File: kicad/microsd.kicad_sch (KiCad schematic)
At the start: 3 parts, among them J4 Micro_SD_Card_Det1

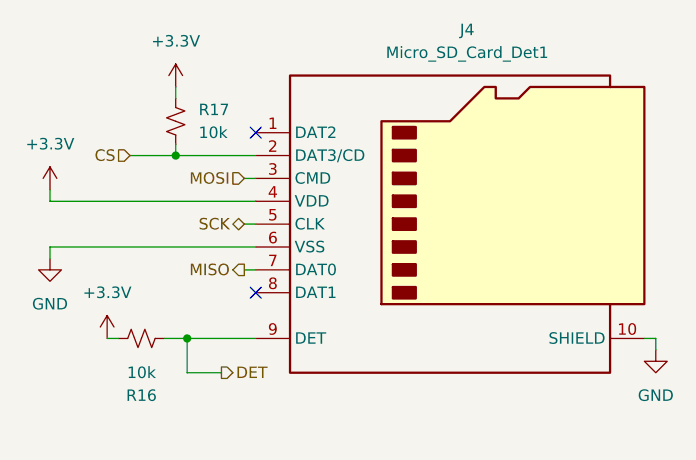
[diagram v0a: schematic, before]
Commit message: finish pcb
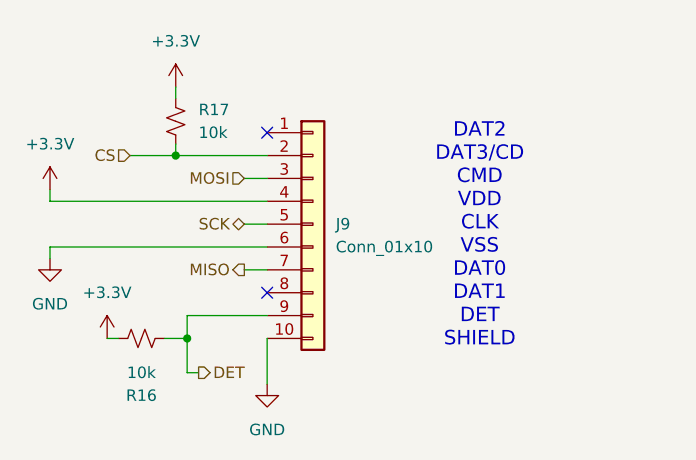
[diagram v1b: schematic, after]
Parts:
- removed J4: Micro_SD_Card_Det1, symbol Connector:Micro_SD_Card_Det1
- added J9: Conn_01x10, Connector_PinSocket_2.54mm:PinSocket_1x10_P2.54mm_Vertical, symbol Connector_Generic:Conn_01x10
- R16, R17: footprint (none) -> Resistor_THT:R_Axial_DIN0207_L6.3mm_D2.5mm_P10.16mm_Horizontal
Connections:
- net +3.3V: now also J9.4 (Pin_4)
- net CS: now also J9.2 (Pin_2)
- net DET: now also J9.9 (Pin_9)
- net GND: now also J9.10 (Pin_10), J9.6 (Pin_6)
- net MISO: now also J9.7 (Pin_7)
- net MOSI: now also J9.3 (Pin_3)
- net SCK: now also J9.5 (Pin_5)
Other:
- note added: "DAT2 DAT3/CD CMD VDD CLK VSS DAT0 DAT1 DET SHIELD"
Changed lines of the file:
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@@
 	(generator_version "9.0")
 	(paper "A4")
+	(text "DAT2\nDAT3/CD\nCMD\nVDD\nCLK\nVSS\nDAT0\nDAT1\nDET\nSHIELD"
+		(exclude_from_sim no)
+		(at 238.252 59.69 0)
+		(effects
+			(font
+				(size 1.6002 1.6002)
+			)
+		)
+	)
 	(junction
 		(at 204.47 50.8)
@@
 	)
 	(no_connect
-		(at 213.36 48.26)
+		(at 214.63 48.26)
 	)
 	(no_connect
-		(at 213.36 66.04)
-	)
-	(wire
-		(pts
-			(xy 257.81 71.12) (xy 256.54 71.12)
-		)
-		(stroke
-			(width 0)
-			(type default)
-		)
-	)
-	(wire
-		(pts
-			(xy 190.5 60.96) (xy 213.36 60.96)
+		(at 214.63 66.04)
+	)
+	(wire
+		(pts
+			(xy 190.5 60.96) (xy 214.63 60.96)
+		)
+		(stroke
+			(width 0)
+			(type default)
+		)
+	)
+	(wire
+		(pts
+			(xy 205.74 68.58) (xy 205.74 71.12)
 		)
 		(stroke
@@
 	(wire
 		(pts
-			(xy 204.47 50.8) (xy 213.36 50.8)
+			(xy 204.47 50.8) (xy 214.63 50.8)
 		)
 		(stroke
@@
 	(wire
 		(pts
-			(xy 212.09 58.42) (xy 213.36 58.42)
-		)
-		(stroke
-			(width 0)
-			(type default)
-		)
-	)
-	(wire
-		(pts
-			(xy 190.5 55.88) (xy 213.36 55.88)
-		)
-		(stroke
-			(width 0)
-			(type default)
-		)
-	)
-	(wire
-		(pts
-			(xy 257.81 72.39) (xy 257.81 71.12)
-		)
-		(stroke
-			(width 0)
-			(type default)
-		)
-	)
-	(wire
-		(pts
-			(xy 212.09 63.5) (xy 213.36 63.5)
+			(xy 212.09 58.42) (xy 214.63 58.42)
+		)
+		(stroke
+			(width 0)
+			(type default)
+		)
+	)
+	(wire
+		(pts
+			(xy 190.5 55.88) (xy 214.63 55.88)
+		)
+		(stroke
+			(width 0)
+			(type default)
+		)
+	)
+	(wire
+		(pts
+			(xy 212.09 63.5) (xy 214.63 63.5)
 		)
 		(stroke
@@
 	(wire
 		(pts
-			(xy 209.55 74.93) (xy 205.74 74.93)
-		)
-		(stroke
-			(width 0)
-			(type default)
-		)
-	)
-	(wire
-		(pts
-			(xy 205.74 71.12) (xy 213.36 71.12)
+			(xy 207.01 74.93) (xy 205.74 74.93)
+		)
+		(stroke
+			(width 0)
+			(type default)
+		)
+	)
+	(wire
+		(pts
+			(xy 214.63 71.12) (xy 214.63 76.2)
+		)
+		(stroke
+			(width 0)
+			(type default)
+		)
+	)
+	(wire
+		(pts
+			(xy 205.74 68.58) (xy 214.63 68.58)
 		)
 		(stroke
@@
 	(wire
 		(pts
-			(xy 212.09 53.34) (xy 213.36 53.34)
+			(xy 212.09 53.34) (xy 214.63 53.34)
 		)
 		(stroke
@@
 	(hierarchical_label "DET"
 		(shape output)
-		(at 209.55 74.93 0)
+		(at 207.01 74.93 0)
 		(effects
 			(font
@@
 	)
 	(symbol
-		(lib_id "Connector:Micro_SD_Card_Det1")
-		(at 236.22 58.42 0)
+		(lib_id "Connector_Generic:Conn_01x10")
+		(at 219.71 58.42 0)
 		(unit 1)
 		(exclude_from_sim no)
@@
 		(dnp no)
 		(fields_autoplaced yes)
-		(property "Reference" "J4"
-			(at 236.855 36.83 0)
-			(effects
-				(font
-					(size 1.27 1.27)
-				)
-			)
-		)
-		(property "Value" "Micro_SD_Card_Det1"
-			(at 236.855 39.37 0)
-			(effects
-				(font
-					(size 1.27 1.27)
-				)
-			)
-		)
-		(property "Footprint" ""
-			(at 288.29 40.64 0)
-			(effects
-				(font
-					(size 1.27 1.27)
-				)
-				(hide yes)
-			)
-		)
-		(property "Datasheet" "https://datasheet.lcsc.com/lcsc/2110151630_XKB-Connectivity-XKTF-015-N_C381082.pdf"
-			(at 236.22 55.88 0)
-			(effects
-				(font
-					(size 1.27 1.27)
-				)
-				(hide yes)
-			)
-		)
-		(property "Description" "Micro SD Card Socket with one card detection pin"
-			(at 236.22 58.42 0)
-			(effects
-				(font
-					(size 1.27 1.27)
-				)
-				(hide yes)
-			)
+		(property "Reference" "J9"
+			(at 222.25 58.4199 0)
+			(effects
+				(font
+					(size 1.27 1.27)
+				)
+				(justify left)
+			)
+		)
+		(property "Value" "Conn_01x10"
+			(at 222.25 60.9599 0)
+			(effects
+				(font
+					(size 1.27 1.27)
+				)
+				(justify left)
+			)
+		)
+		(property "Footprint" "Connector_PinSocket_2.54mm:PinSocket_1x10_P2.54mm_Vertical"
+			(at 219.71 58.42 0)
+			(effects
+				(font
+					(size 1.27 1.27)
+				)
+				(hide yes)
+			)
+		)
+		(property "Datasheet" "~"
+			(at 219.71 58.42 0)
+			(effects
+				(font
+					(size 1.27 1.27)
+				)
+				(hide yes)
+			)
+		)
+		(property "Description" "Generic connector, single row, 01x10, script generated (kicad-library-utils/schlib/autogen/connector/)"
+			(at 219.71 58.42 0)
+			(effects
+				(font
+					(size 1.27 1.27)
+				)
+				(hide yes)
+			)
+		)
+		(pin "10"
+		)
+		(pin "1"
+		)
+		(pin "9"
+		)
+		(pin "7"
+		)
+		(pin "8"
+		)
+		(pin "2"
+		)
+		(pin "5"
 		)
 		(pin "4"
 		)
-		(pin "7"
+		(pin "3"
 		)
 		(pin "6"
-		)
-		(pin "3"
-		)
-		(pin "5"
-		)
-		(pin "8"
-		)
-		(pin "2"
-		)
-		(pin "1"
-		)
-		(pin "9"
-		)
-		(pin "10"
 		)
 		(instances
 			(project ""
 				(path "/78341cab-a048-4351-a366-4c432cce3019/1eb4b5a7-2367-4a58-83ec-1e8dc8470950"
-					(reference "J4")
+					(reference "J9")
 					(unit 1)
 				)
@@
 			)
 		)
-		(property "Footprint" ""
+		(property "Footprint" "Resistor_THT:R_Axial_DIN0207_L6.3mm_D2.5mm_P10.16mm_Horizontal"
 			(at 200.66 71.12 0)
 			(effects
@@
 			)
 		)
-		(property "Footprint" ""
+		(property "Footprint" "Resistor_THT:R_Axial_DIN0207_L6.3mm_D2.5mm_P10.16mm_Horizontal"
 			(at 204.47 46.99 0)
 			(effects
@@
 	(symbol
 		(lib_id "power:GND")
-		(at 257.81 72.39 0)
+		(at 214.63 76.2 0)
 		(unit 1)
 		(exclude_from_sim no)
@@
 		(fields_autoplaced yes)
 		(property "Reference" "#PWR032"
-			(at 257.81 78.74 0)
+			(at 214.63 82.55 0)
 			(effects
 				(font
@@
 		)
 		(property "Value" "GND"
-			(at 257.81 77.47 0)
+			(at 214.63 81.28 0)
 			(effects
 				(font
@@
 		)
 		(property "Footprint" ""
-			(at 257.81 72.39 0)
+			(at 214.63 76.2 0)
 			(effects
 				(font
@@
 		)
 		(property "Datasheet" ""
-			(at 257.81 72.39 0)
+			(at 214.63 76.2 0)
 			(effects
 				(font
@@
 		)
 		(property "Description" "Power symbol creates a global label with name \"GND\" , ground"
-			(at 257.81 72.39 0)
-			(effects
-				(font
+			(at 214.63 76.2 0)
+			(effects
+				(font
